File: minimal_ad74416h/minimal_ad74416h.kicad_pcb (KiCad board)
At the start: 4 copper layers, 25.4 x 25.4 mm, 1 part, among them U1 AD74416HBCPZ-RL7

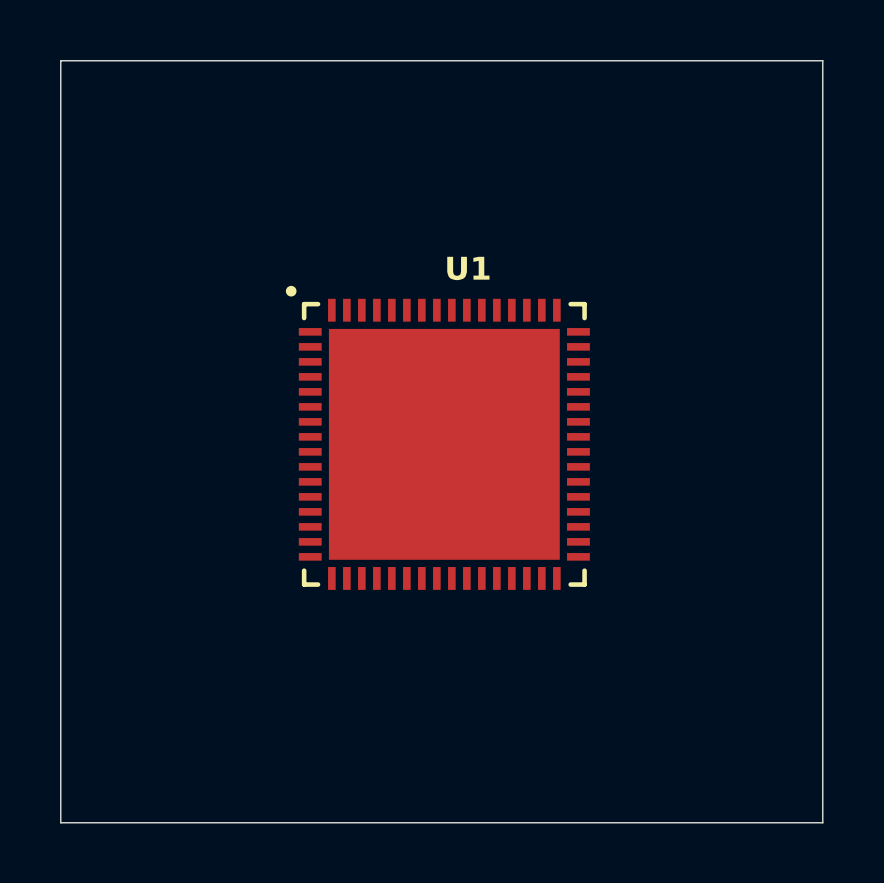
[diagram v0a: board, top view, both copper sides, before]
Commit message: minor changes
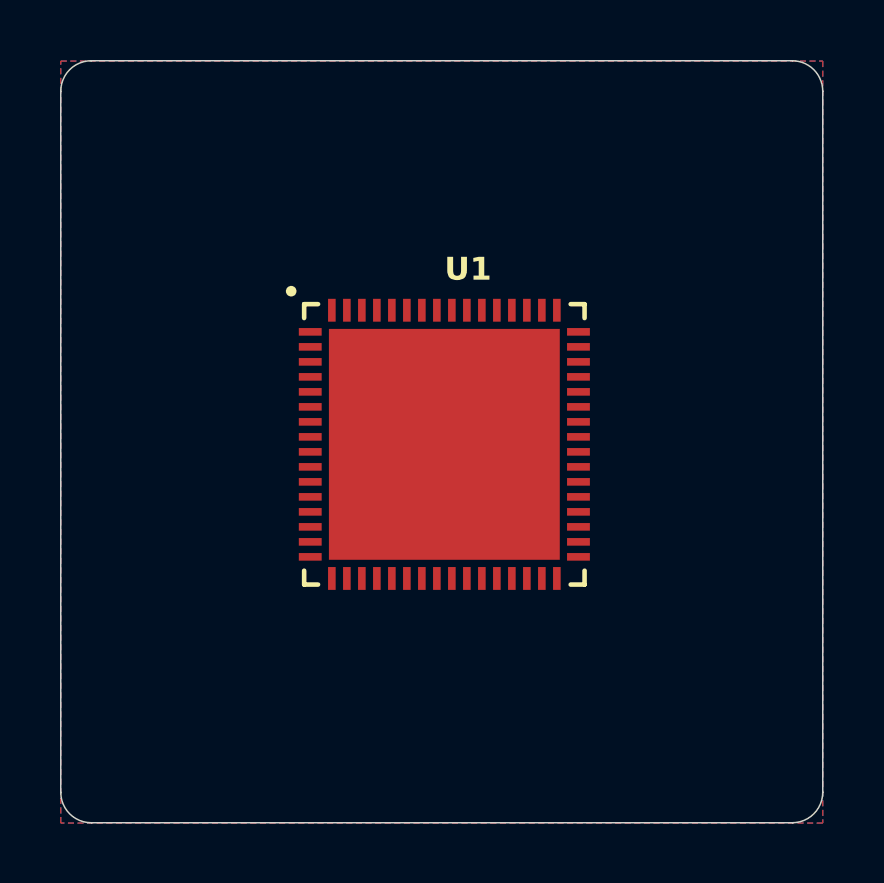
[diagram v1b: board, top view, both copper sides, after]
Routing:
- added copper zone on B.Cu, net (none)
- added copper zone on F.Cu, net (none)
- added copper zone on In1.Cu, net (none)
- added copper zone on In2.Cu, net (none)
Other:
- outline, holes or cut-outs redrawn
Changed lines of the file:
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@@
 		)
 	)
-	(gr_rect
-		(start 122.682 100.624087)
-		(end 148.082 126.024087)
+	(gr_arc
+		(start 147.066 100.624087)
+		(mid 147.784425 100.921666)
+		(end 148.082 101.640087)
 		(stroke
 			(width 0.05)
-			(type solid)
+			(type default)
 		)
-		(fill no)
 		(layer "Edge.Cuts")
 	)
+	(gr_line
+		(start 122.682 125.008087)
+		(end 122.682 101.640087)
+		(stroke
+			(width 0.05)
+			(type default)
+		)
+		(layer "Edge.Cuts")
+	)
+	(gr_line
+		(start 148.082 101.640087)
+		(end 148.082 125.008087)
+		(stroke
+			(width 0.05)
+			(type default)
+		)
+		(layer "Edge.Cuts")
+	)
+	(gr_arc
+		(start 123.698 126.024087)
+		(mid 122.979584 125.726507)
+		(end 122.682 125.008087)
+		(stroke
+			(width 0.05)
+			(type default)
+		)
+		(layer "Edge.Cuts")
+	)
+	(gr_arc
+		(start 122.682 101.640087)
+		(mid 122.97958 100.921667)
+		(end 123.698 100.624087)
+		(stroke
+			(width 0.05)
+			(type default)
+		)
+		(layer "Edge.Cuts")
+	)
+	(gr_line
+		(start 147.066 126.024087)
+		(end 123.698 126.024087)
+		(stroke
+			(width 0.05)
+			(type default)
+		)
+		(layer "Edge.Cuts")
+	)
+	(gr_arc
+		(start 148.082 125.008087)
+		(mid 147.78442 125.726507)
+		(end 147.066 126.024087)
+		(stroke
+			(width 0.05)
+			(type default)
+		)
+		(layer "Edge.Cuts")
+	)
+	(gr_line
+		(start 123.698 100.624087)
+		(end 147.066 100.624087)
+		(stroke
+			(width 0.05)
+			(type default)
+		)
+		(layer "Edge.Cuts")
+	)
+	(zone
+		(net 0)
+		(net_name "")
+		(layers "F.Cu" "B.Cu" "In1.Cu" "In2.Cu")
+		(hatch none 0.508)
+		(connect_pads
+			(clearance 0.508)
+		)
+		(min_thickness 0.508)
+		(filled_areas_thickness no)
+		(fill yes
+			(thermal_gap 0.508)
+			(thermal_bridge_width 0.508)
+			(smoothing fillet)
+			(radius 0.508)
+			(island_removal_mode 1)
+			(island_area_min 9.999999)
+		)
+		(polygon
+			(pts
+				(xy 122.682 100.6348) (xy 148.082 100.6348) (xy 148.082 126.0348) (xy 122.682 126.0348)
+			)
+		)
+	)
 	(embedded_fonts no)
